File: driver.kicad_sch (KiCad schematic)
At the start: 23 parts, among them U12 SN75107, U13 SN75110, U15 SN75110, U16 SN75110, U17 SN75110, U18 SN75110, U19 SN75110, U9 SN75107

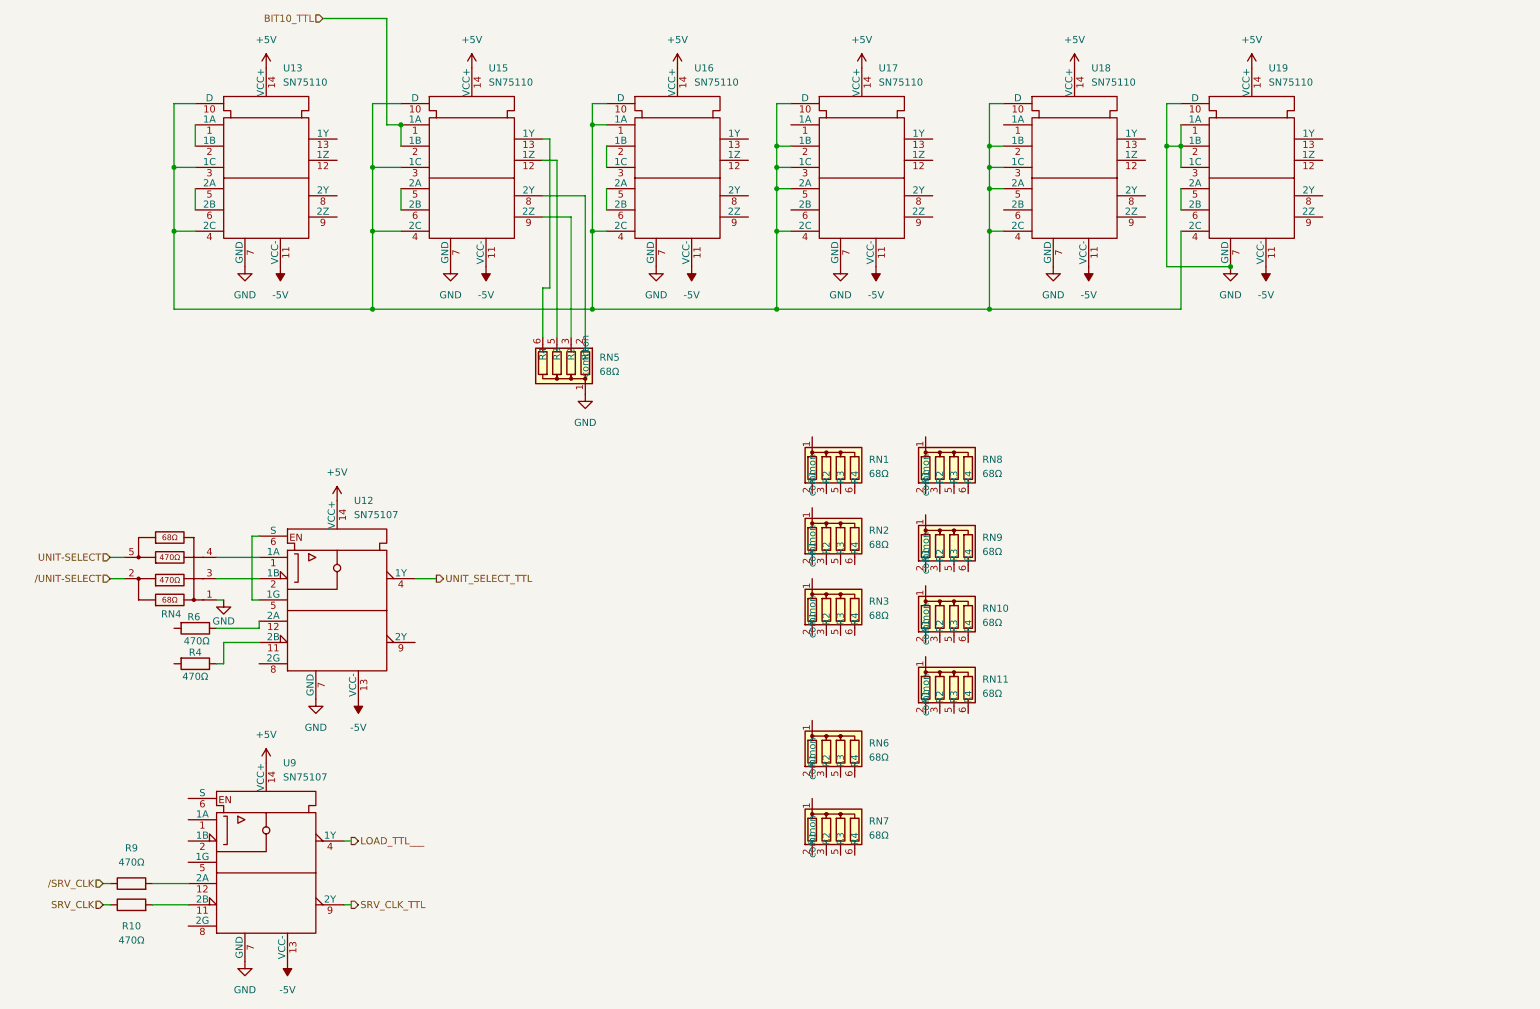
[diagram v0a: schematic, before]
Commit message: weitere verdrahtungen nachvollzogen
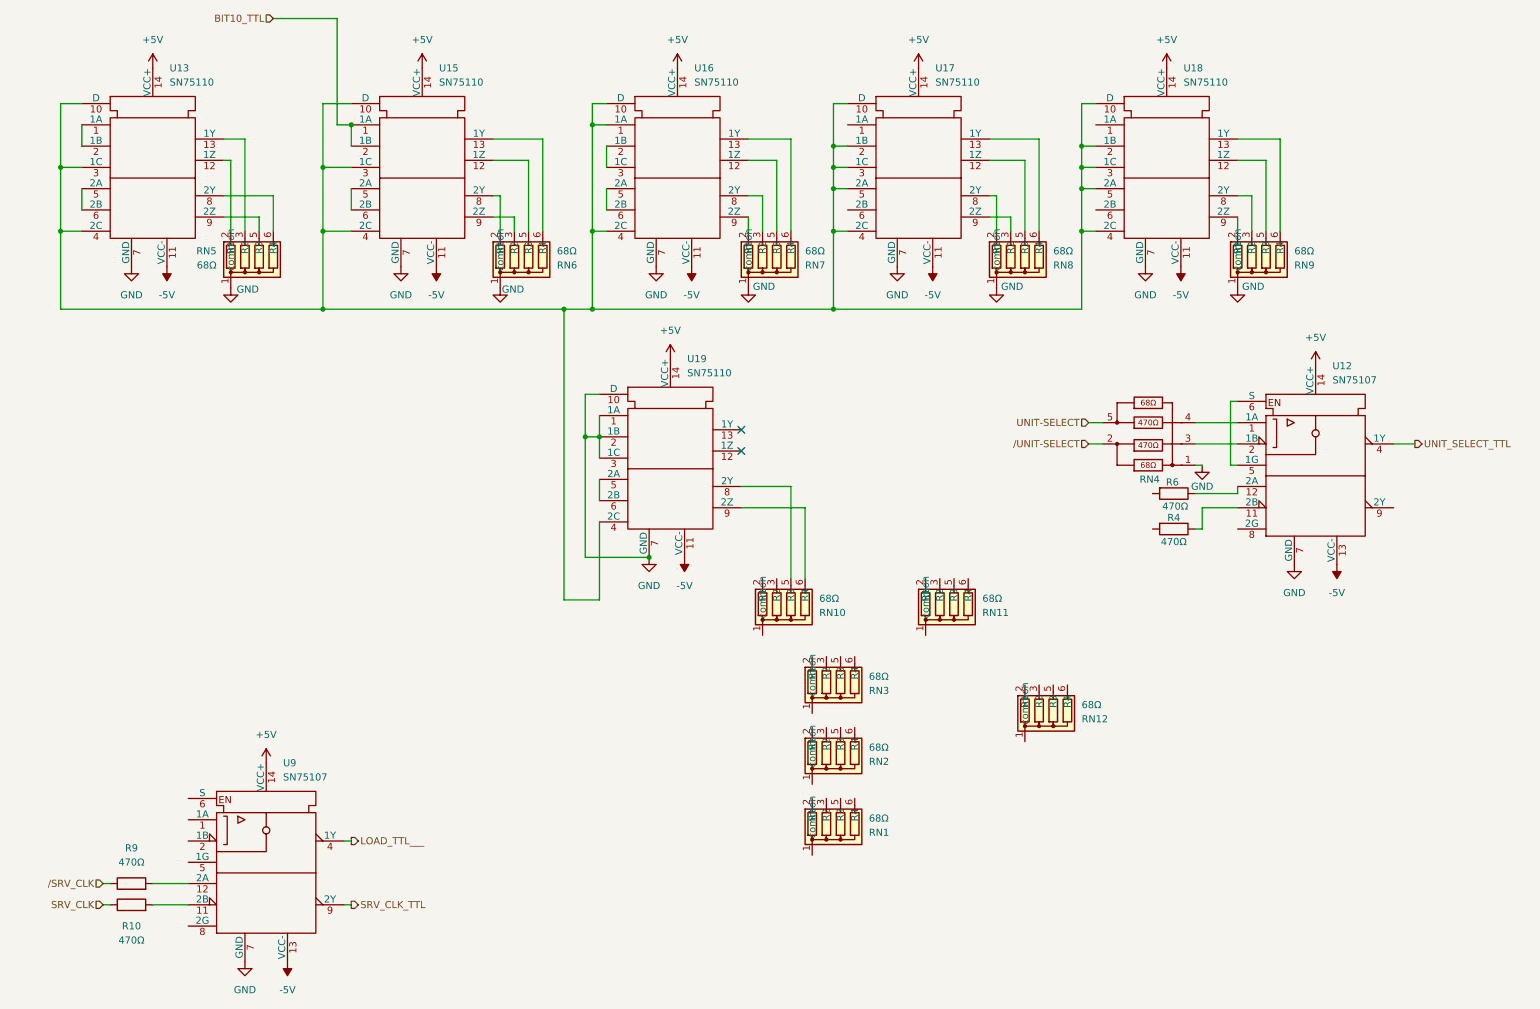
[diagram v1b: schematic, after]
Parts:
- added RN12: 68Ω, Resistor_THT:R_Array_SIP6, symbol line termination resistors:3553
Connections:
- net GND: now also RN6.1 (common), RN7.1 (common), RN8.1 (common), RN9.1 (common)
- net at RN9.2 (R1): now also U18.9 (2Z)
- net at RN9.3 (R2): now also U18.8 (2Y)
- net at RN9.5 (R3): now also U18.12 (1Z)
- net at RN9.6 (R4): now also U18.13 (1Y)
- net at RN8.2 (R1): now also U17.8 (2Y)
- net at RN8.3 (R2): now also U17.9 (2Z)
- net at RN8.5 (R3): now also U17.12 (1Z)
- net at RN8.6 (R4): now also U17.13 (1Y)
- net at U13.12 (1Z): now also RN5.2 (R1)
- net at U13.13 (1Y): now also RN5.3 (R2)
- net at U13.8 (2Y): now also RN5.6 (R4)
- net at U13.9 (2Z): now also RN5.5 (R3)
- net at U15.8 (2Y): now also RN6.2 (R1); no longer RN5.2 (R1)
- net at U15.9 (2Z): now also RN6.3 (R2); no longer RN5.3 (R2)
- net at U15.12 (1Z): now also RN6.5 (R3); no longer RN5.5 (R3)
- net at U15.13 (1Y): now also RN6.6 (R4); no longer RN5.6 (R4)
- net at U16.12 (1Z): now also RN7.5 (R3)
- net at U16.13 (1Y): now also RN7.6 (R4)
- net at U16.8 (2Y): now also RN7.3 (R2)
- net at U16.9 (2Z): now also RN7.2 (R1)
- net at U19.8 (2Y): now also RN10.5 (R3)
- net at U19.9 (2Z): now also RN10.6 (R4)
- no-connect marks 0 -> 2
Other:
- moved on the sheet: R4, R6, RN1, RN10, RN11, RN2, RN3, RN4, RN6, RN7, RN8, RN9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
